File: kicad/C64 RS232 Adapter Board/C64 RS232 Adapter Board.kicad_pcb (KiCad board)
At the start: 2 copper layers, 29 parts, among them J1 RS232_HDR, J2 DB25_RS232, J3 C64_USER_PORT, J4 User Port Breakout, SW1 RESET, U1 MAX3241ECAI+T

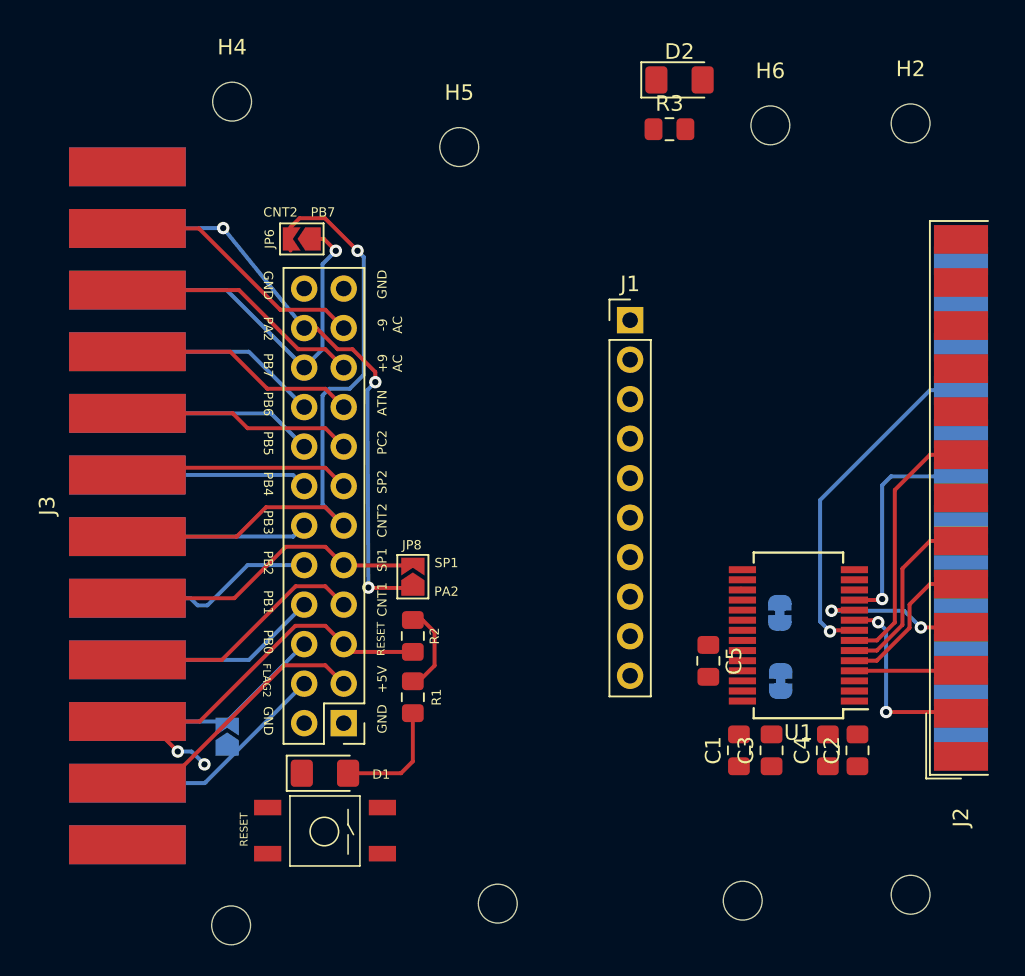
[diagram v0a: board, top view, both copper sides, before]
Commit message: First layout done
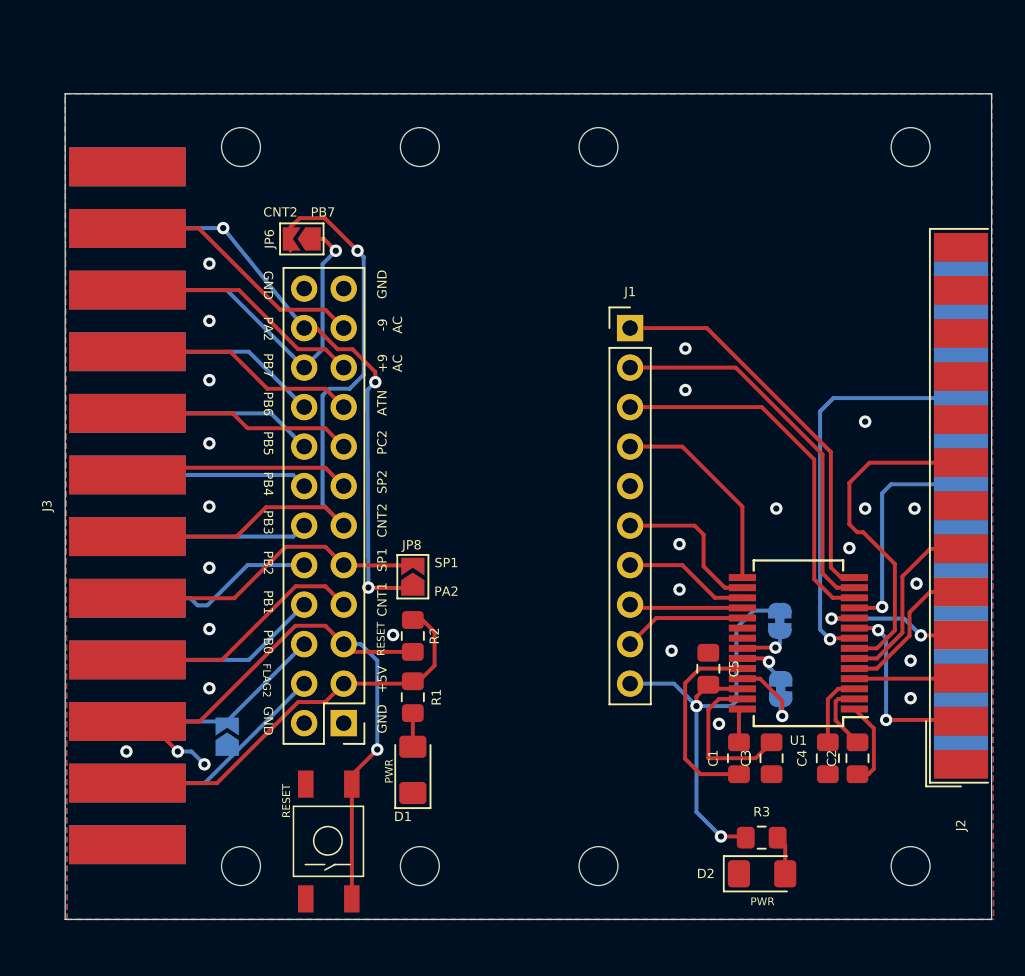
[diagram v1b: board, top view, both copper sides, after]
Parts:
- moved D2 51.3 mm to (89.0, 103.6)
- moved R3 45.9 mm to (89.0, 101.3)
- moved H6 11.1 mm to (78.5, 56.9)
- moved H8 9.53 mm to (78.5, 103.1)
- moved D1 5.66 mm to (66.5, 96.9), turned to 90 degrees
- moved H7 5.56 mm to (67.0, 103.1)
- moved H1 3.86 mm to (55.5, 103.1)
- moved H4 2.98 mm to (55.5, 56.9)
- moved H5 2.53 mm to (67.0, 56.9), turned to 45 degrees
- moved H3 1.84 mm to (98.6, 103.1)
- moved H2 1.52 mm to (98.6, 56.9)
- moved SW1 0.63 mm to (61.1, 101.5), turned to 180 degrees
- moved C1 0.51 mm to (87.5, 96.2)
- moved C2 0.51 mm to (95.1, 96.2)
- moved C3 0.51 mm to (89.6, 96.2)
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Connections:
- J1 pad 10: (no net) -> +5V
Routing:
- net +5V: track 29.2 -> 63.1 mm, vias 0 -> 2
- net /TXD_TTL: track 0.00 -> 25.4 mm
- net /DTR_TTL: track 0.00 -> 24.8 mm
- net /RTS_TTL: track 0.00 -> 24.0 mm
- net /RESET: track 31.1 -> 50.3 mm, vias 2 -> 3
- net /RI_TTL: track 0.00 -> 13.4 mm
- net Net-(C1-Pad1): track 0.00 -> 12.8 mm
- net Net-(C3-Pad2): track 0.00 -> 10.1 mm
- net /DCD_TTL: track 0.00 -> 10.1 mm
- net /DSR_TTL: track 0.13 -> 8.22 mm
- net /RXD_TTL: track 0.00 -> 7.92 mm
- net /CTS_TTL: track 0.00 -> 7.31 mm
- net Net-(C2-Pad1): track 0.00 -> 5.56 mm
- net Net-(D1-Pad2): track 7.58 -> 2.16 mm
- net GND: track 0.00 -> 5.25 mm, vias 0 -> 16
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- added copper zone on B.Cu, net GND
- added copper zone on F.Cu, net GND
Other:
- board outline added: 59.6 x 53.1 mm
- board text added: "PWR"
